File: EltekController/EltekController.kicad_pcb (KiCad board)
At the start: 2 copper layers, 65 x 37.5 mm, 36 parts, among them J1 CANBUS, J2 ESP-PROG, J3 Qwiic, SW1 RST, SW2 BOOT, SW3 LEFT, SW4 SEL, SW5 RIGHT, U1 ESP32-S2-WROVER, U2 MAX3051ESA, U3 XC6220B331MR

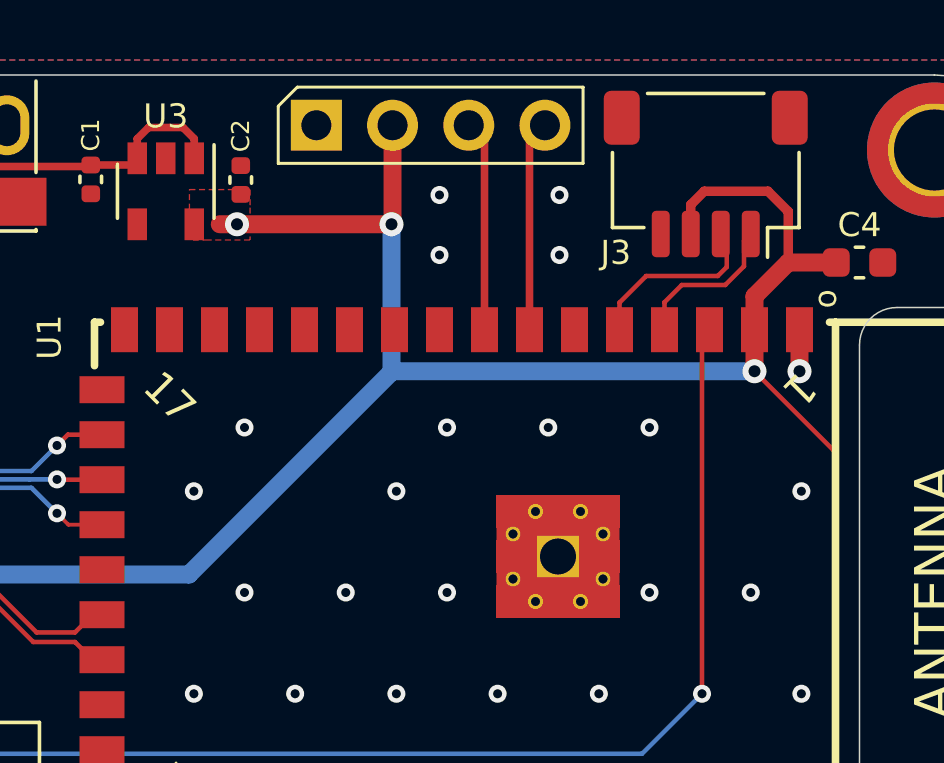
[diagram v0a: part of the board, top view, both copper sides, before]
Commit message: flip VCC and GND on the OLED... sigh
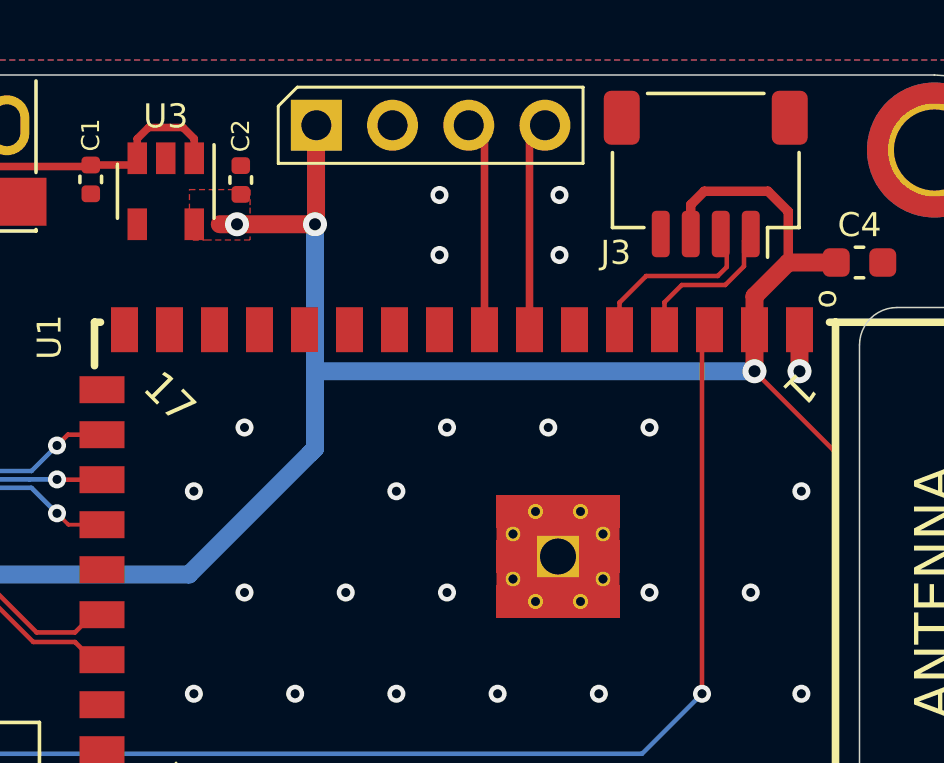
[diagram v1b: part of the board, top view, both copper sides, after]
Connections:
- I2C1 pad 1: GND -> +3V3
- I2C1 pad 2: +3V3 -> GND
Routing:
- net +3V3: track 126.9 -> 128.7 mm

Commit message: Revert "flip VCC and GND on the OLED... sigh"
This reverts commit 16d08c3f3e759163bdd9650e3550ba9f731368f2.
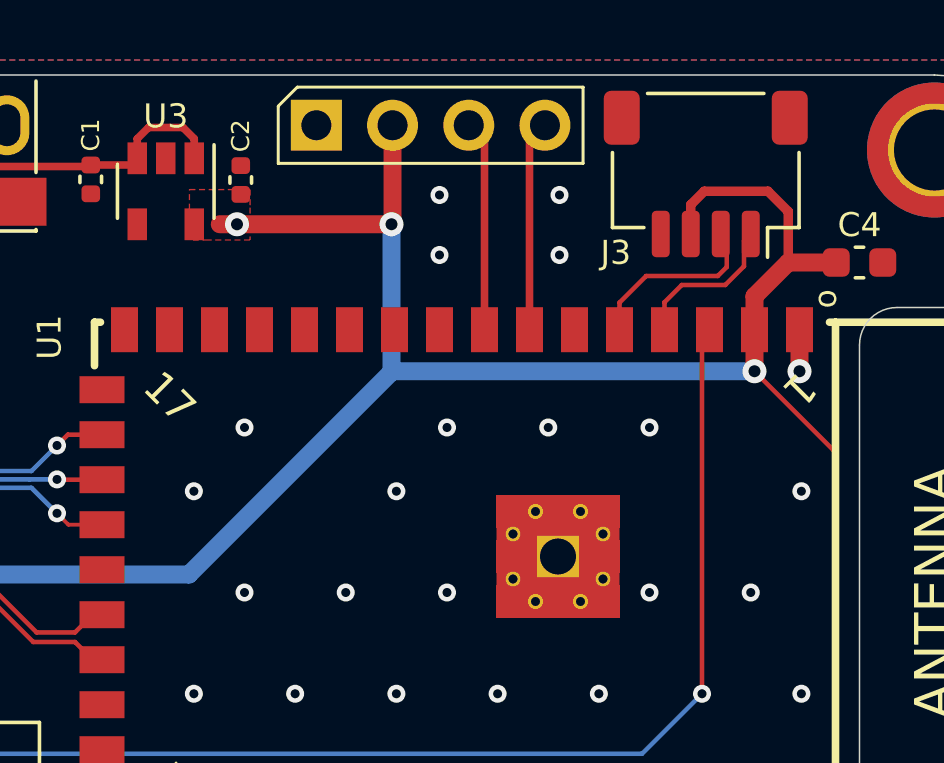
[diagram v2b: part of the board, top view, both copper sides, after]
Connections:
- I2C1 pad 1: +3V3 -> GND
- I2C1 pad 2: GND -> +3V3
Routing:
- net +3V3: track 128.7 -> 126.9 mm
